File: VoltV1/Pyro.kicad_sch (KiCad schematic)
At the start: 13 parts, among them Q1 STL66DN3LLH5, U10 MCP1416T-E_OT, U11 MCP1416T-E_OT

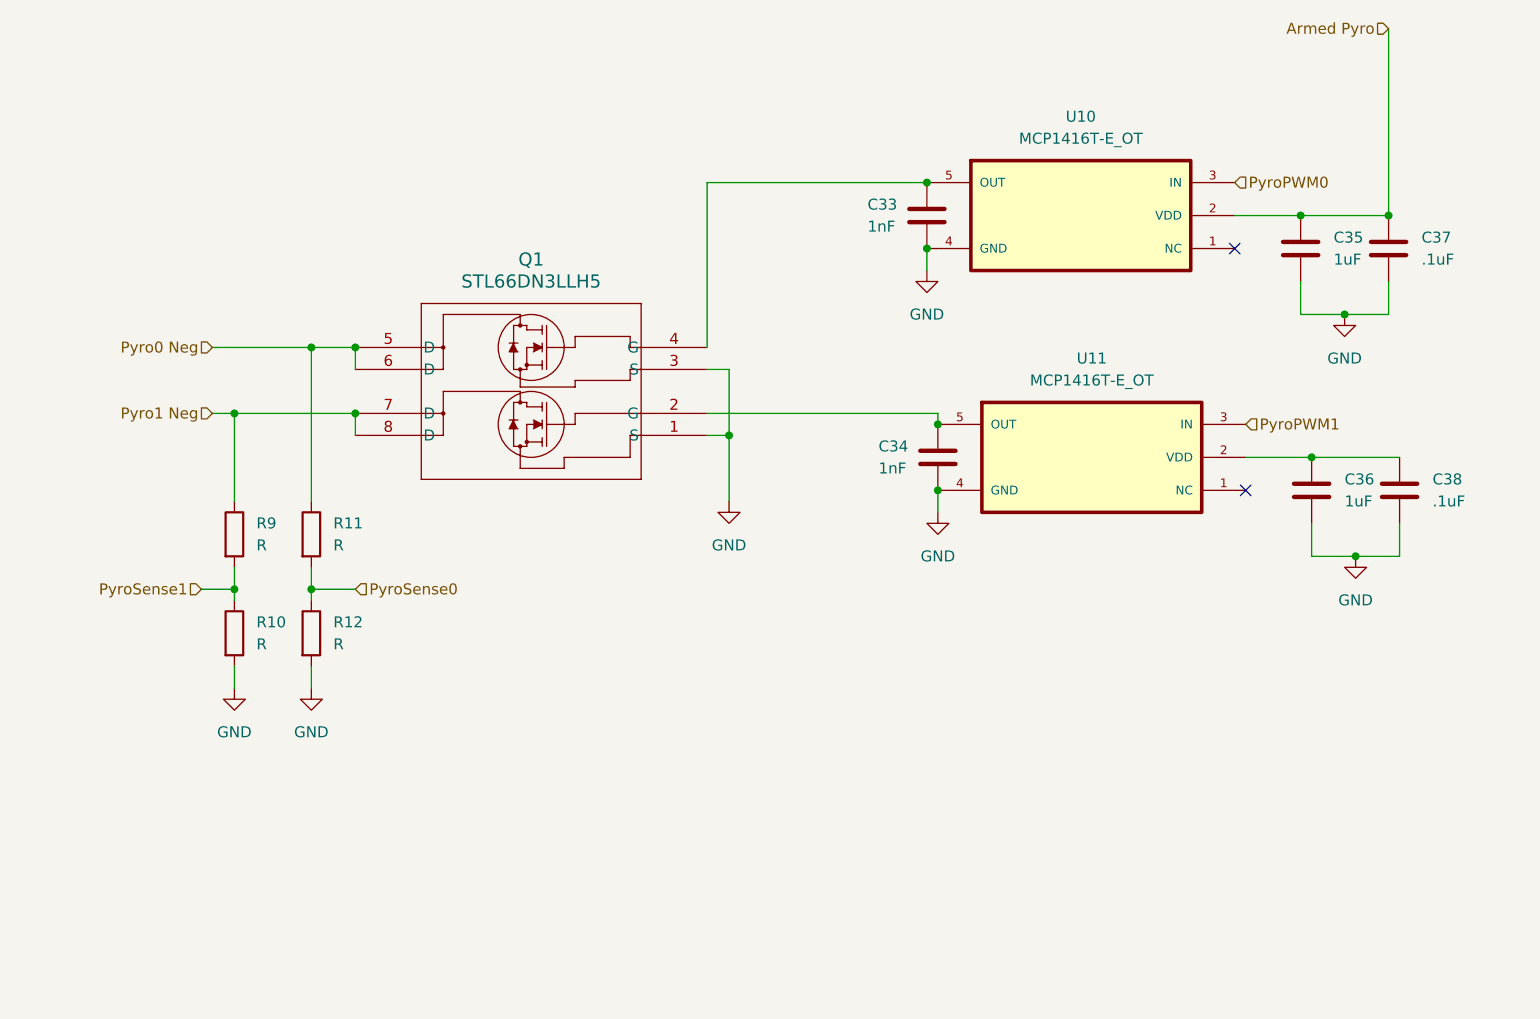
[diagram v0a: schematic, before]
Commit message: merging. power stuff incomplete
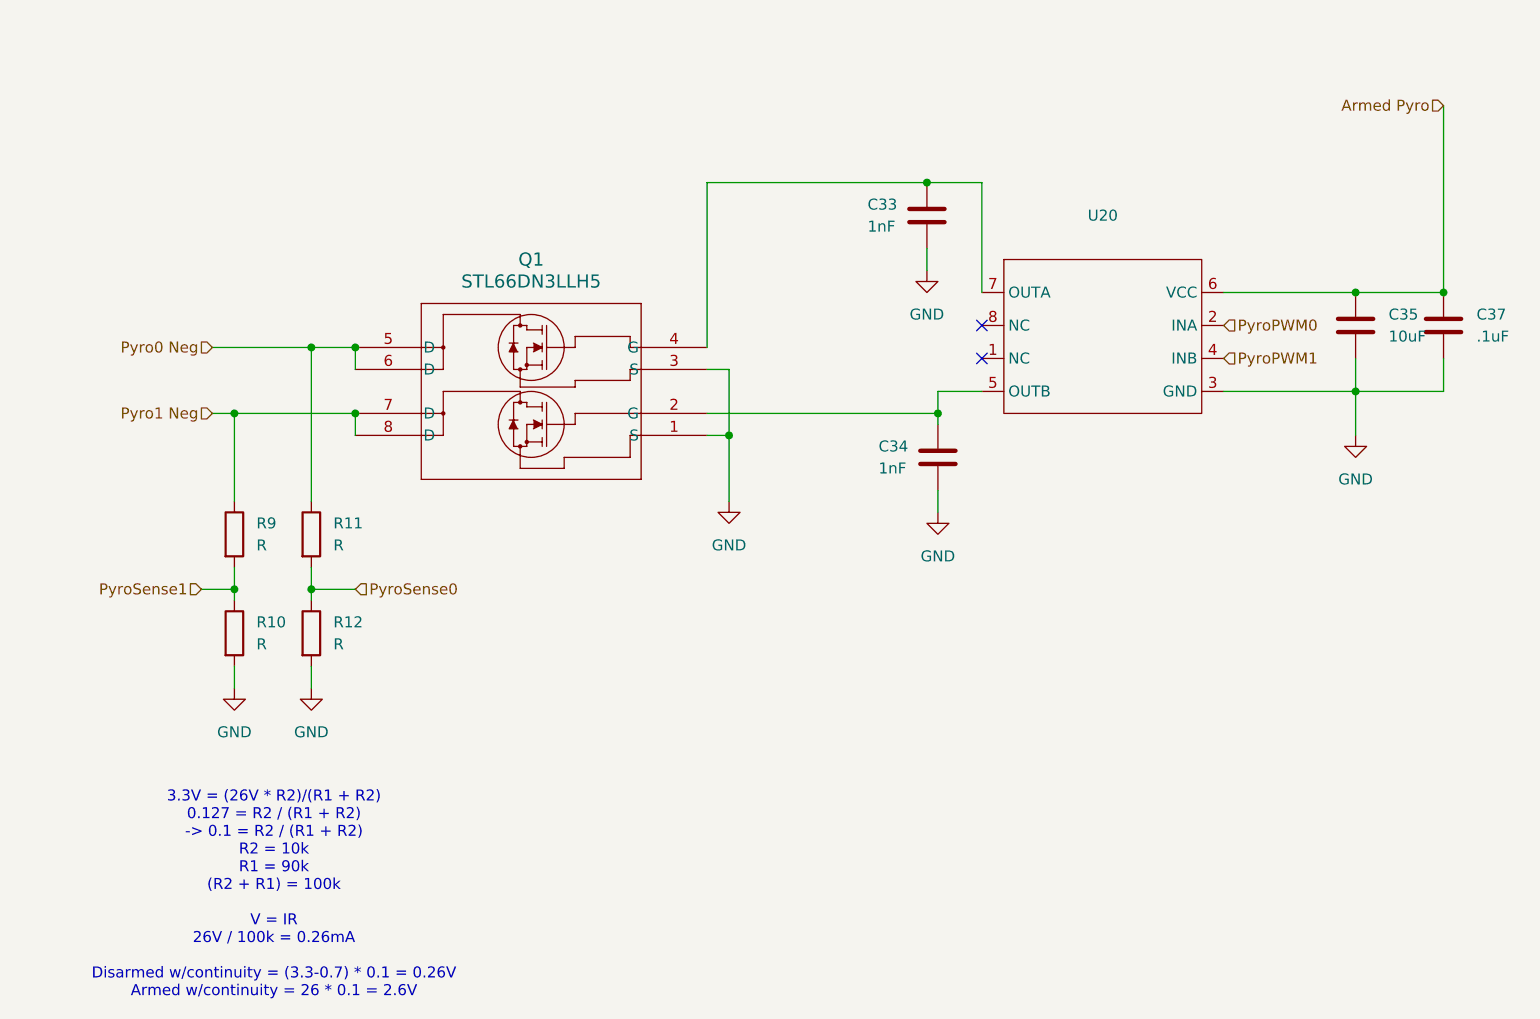
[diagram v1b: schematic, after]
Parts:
- removed C36: 1uF, symbol Device:C
- removed C38: .1uF, symbol Device:C
- removed U10, U11: MCP1416T-E_OT, VOLTV1:SOT95P270X145-5N, symbol VOLTV1:MCP1416T-E_OT
- added U20: ~, Package_SO:SOIC-8_3.9x4.9mm_P1.27mm, symbol VOLTV1:IX4427NTR
- C35: value 1uF -> 10uF
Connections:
- net Armed Pyro: now also U20.6 (VCC)
- net GND: now also U20.3 (GND)
- net PyroPWM0: now also U20.2 (INA)
- net PyroPWM1: now also U20.4 (INB)
- net at C33.2, Q1.4 (G): now also U20.7 (OUTA)
- net at C34.2, Q1.2 (G): now also U20.5 (OUTB)
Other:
- note added: "3.3V = (26V * R2)/(R1 + R2) 0.127 = R2 / (R1 + R2) -> 0.1 = R2 / (R1 + R2) R2 = 10k R1 = 90k (R2 + R1) = 100k V = IR 26V / 100k = 0.26mA Disarmed w/continuity = (3.3-0.7) * 0.1 = 0.26V Armed w/continuity = 26 * 0.1 = 2.6V"
- moved on the sheet: C35, C37

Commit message: schematic updates
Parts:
- C33, C34, C35, C37: footprint (none) -> Capacitor_SMD:C_0402_1005Metric
- R10, R11, R12, R9: footprint (none) -> Resistor_SMD:R_0402_1005Metric
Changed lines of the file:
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@@
 			)
 		)
-		(property "Footprint" ""
+		(property "Footprint" "Capacitor_SMD:C_0402_1005Metric"
 			(at 180.0352 67.31 0)
 			(effects
@@
 			)
 		)
-		(property "Footprint" ""
+		(property "Footprint" "Resistor_SMD:R_0402_1005Metric"
 			(at 56.642 99.06 90)
 			(effects
@@
 			)
 		)
-		(property "Footprint" ""
+		(property "Footprint" "Resistor_SMD:R_0402_1005Metric"
 			(at 47.752 87.63 90)
 			(effects
@@
 			)
 		)
-		(property "Footprint" ""
+		(property "Footprint" "Resistor_SMD:R_0402_1005Metric"
 			(at 56.642 87.63 90)
 			(effects
@@
 			)
 		)
-		(property "Footprint" ""
+		(property "Footprint" "Capacitor_SMD:C_0402_1005Metric"
 			(at 129.8448 74.93 0)
 			(effects
@@
 			)
 		)
-		(property "Footprint" ""
+		(property "Footprint" "Resistor_SMD:R_0402_1005Metric"
 			(at 47.752 99.06 90)
 			(effects
@@
 			)
 		)
-		(property "Footprint" ""
+		(property "Footprint" "Capacitor_SMD:C_0402_1005Metric"
 			(at 128.5748 46.99 0)
 			(effects
@@
 			)
 		)
-		(property "Footprint" ""
+		(property "Footprint" "Capacitor_SMD:C_0402_1005Metric"
 			(at 190.1952 67.31 0)
 			(effects
